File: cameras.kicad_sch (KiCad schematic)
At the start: 30 parts

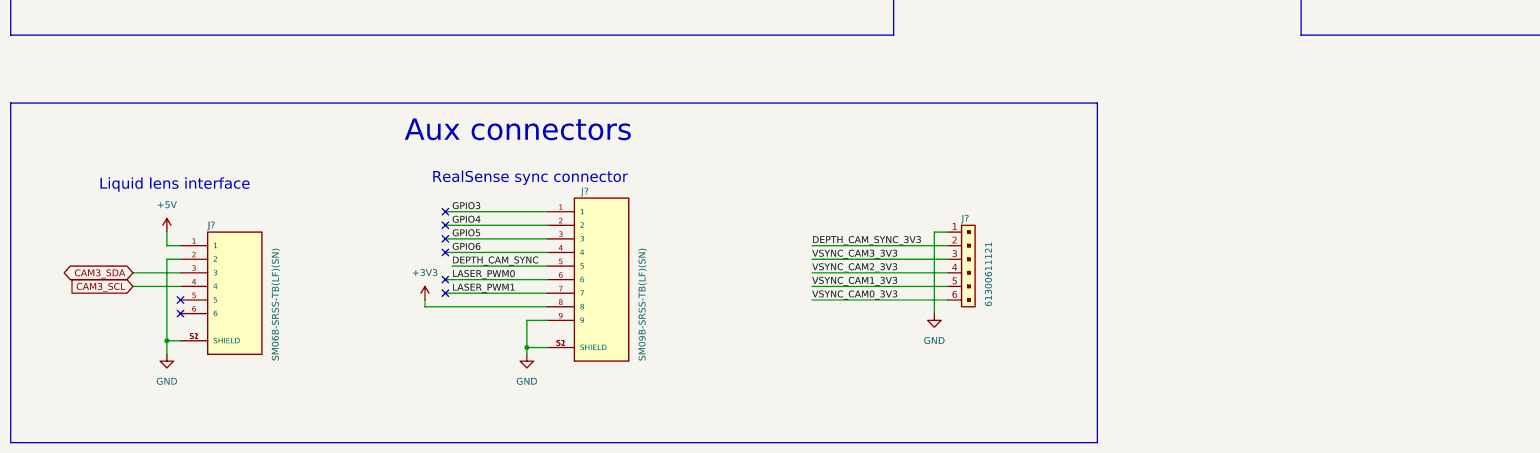
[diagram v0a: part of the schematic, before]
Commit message: Fixes suggested in review
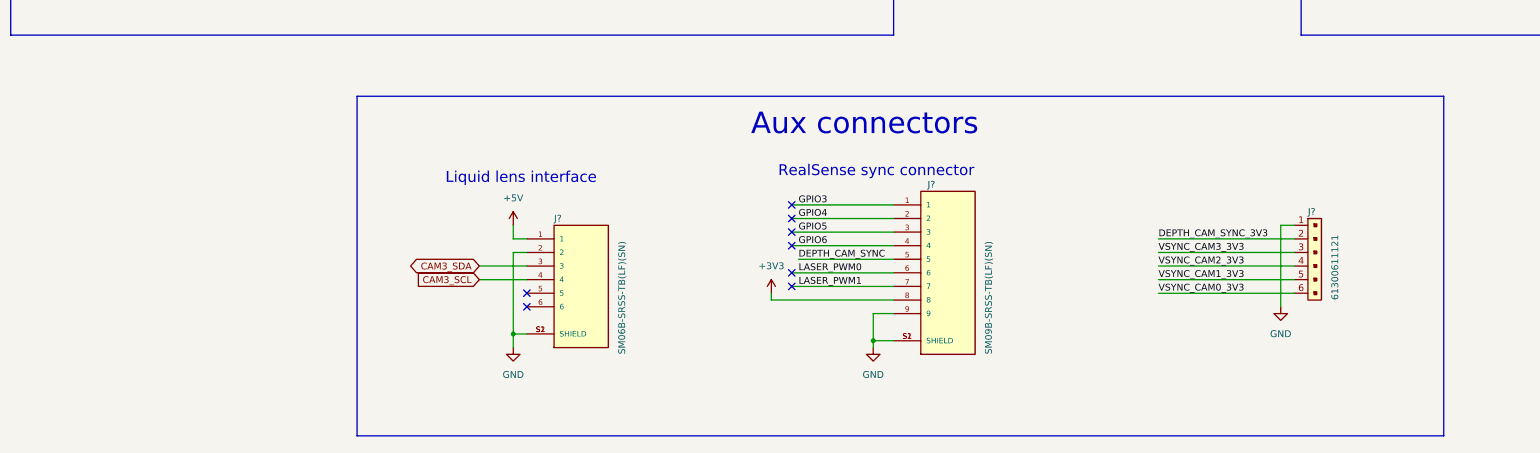
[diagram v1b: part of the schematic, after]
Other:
- moved on the sheet: J?
